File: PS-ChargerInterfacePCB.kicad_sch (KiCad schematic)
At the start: 32 parts, among them J2 LV_Elcon_Connector, J4 BPSConn, J5 Estop 2, J6 Estop 3, K2 Relay_SPST-NC

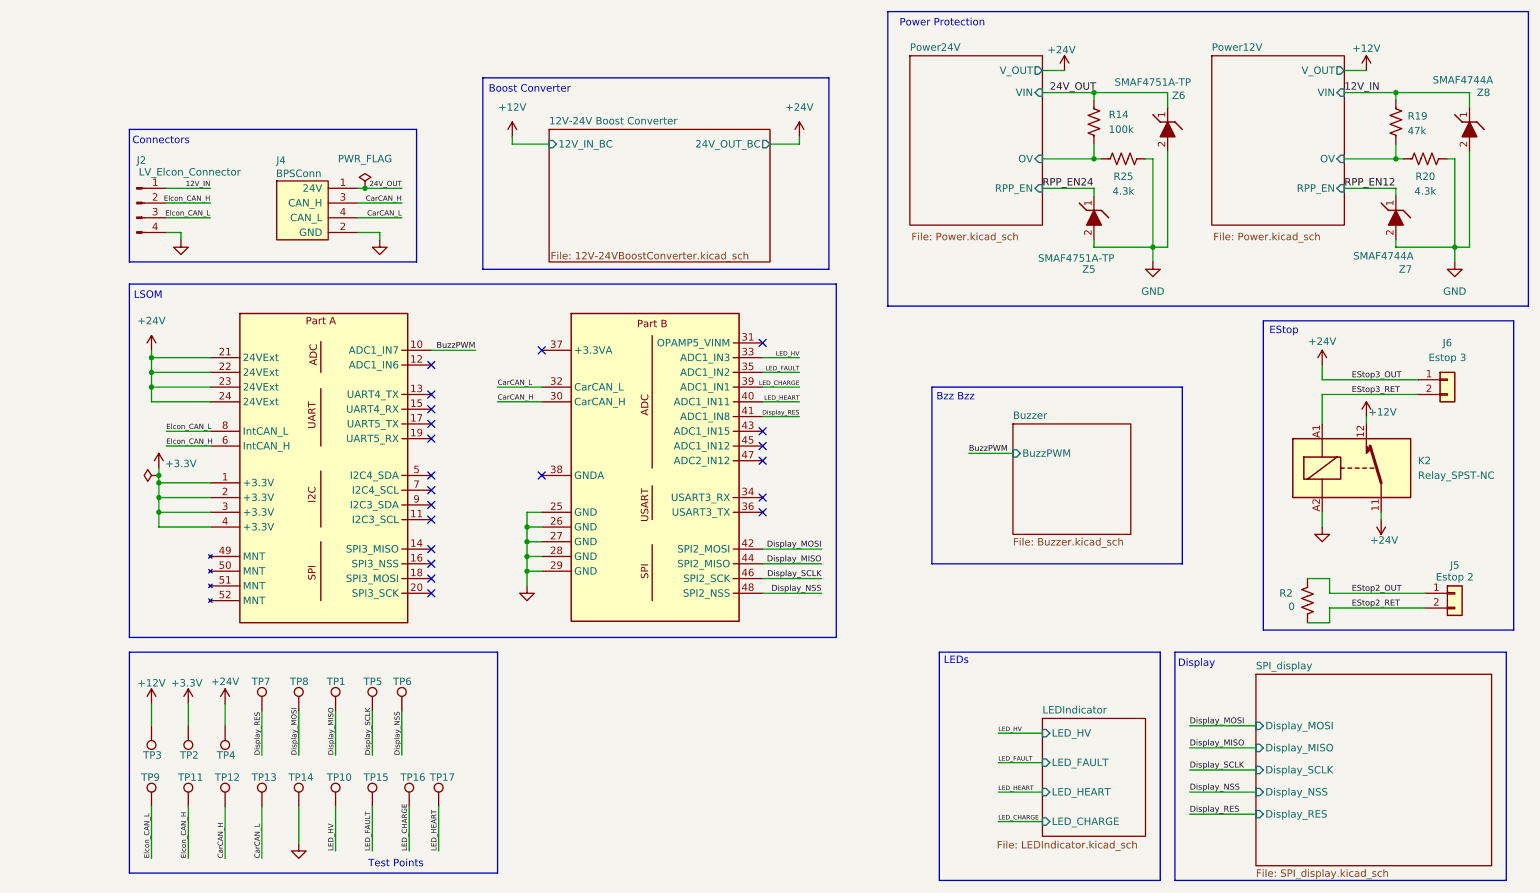
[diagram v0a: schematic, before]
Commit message: RevA5
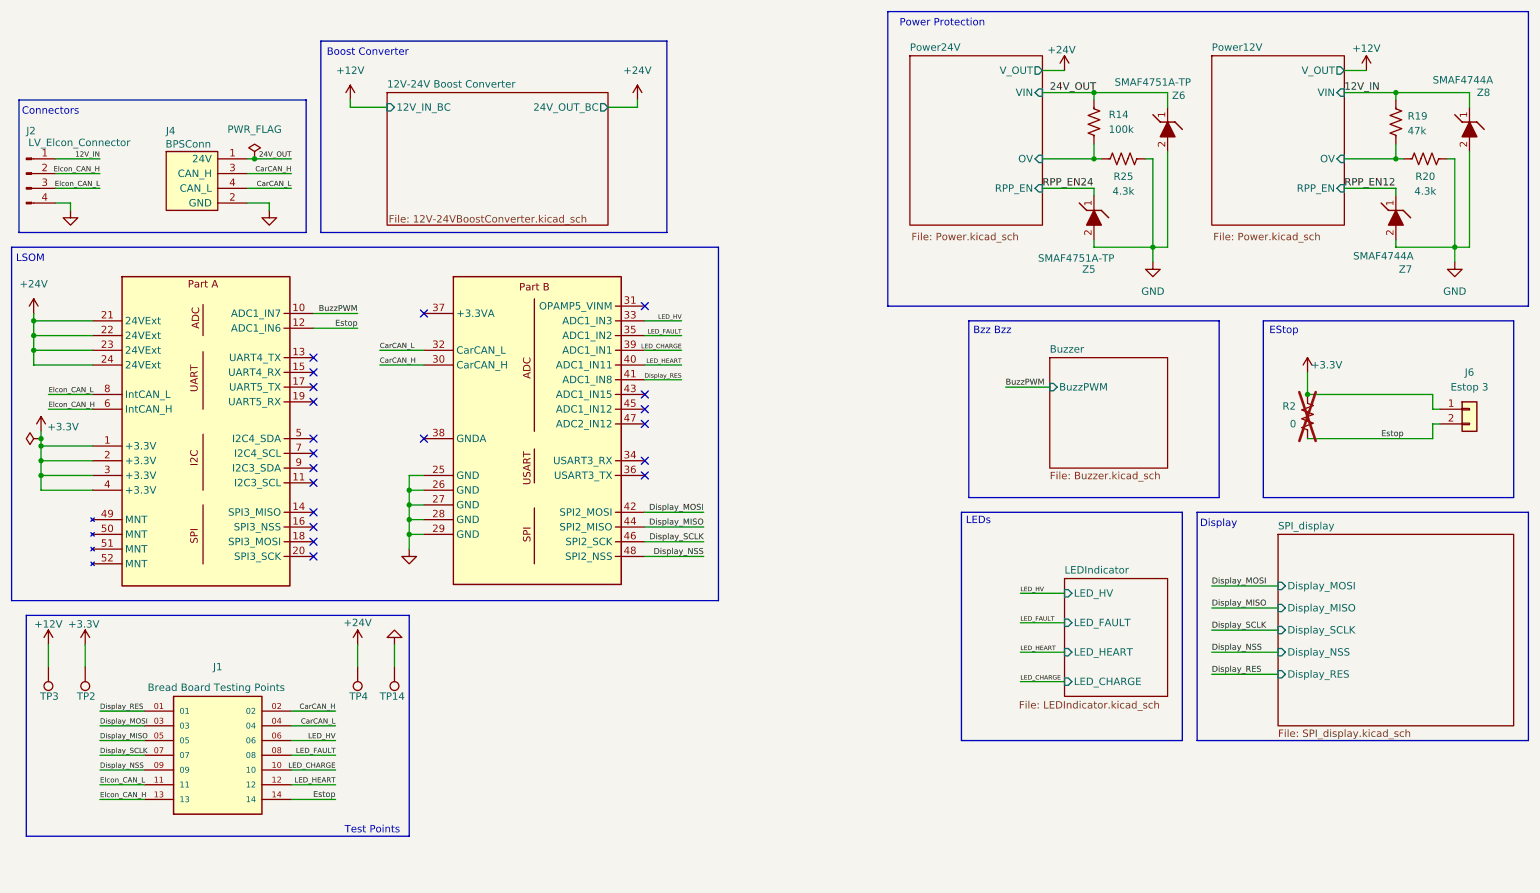
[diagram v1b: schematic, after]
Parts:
- removed J5: Estop 2, symbol Connector_Generic:Conn_01x02
- removed K2: Relay_SPST-NC, symbol Relay:Relay_SPST-NC
- removed TP1, TP10, TP11, TP12, TP13, TP15, TP16, TP17, TP5, TP6, TP7, TP8, TP9: TestPoint, symbol Connector:TestPoint
- added J1: Bread Board Testing Points, SSW-107-21-G-D:SAMTEC_SSW-107-21-G-D, symbol SSW-107-21-G-D:SSW-107-21-G-D
- R2: footprint (none) -> Resistor_SMD:R_0402_1005Metric; now not fitted
- TP14, TP2, TP3, TP4: footprint (none) -> UTSVT_Special:TestPoint_HEX_3mmID
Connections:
- net EStop2_OUT is gone; now on net +3.3V: R2.1
- net EStop2_RET is gone; now on net Estop: R2.2
- net EStop3_RET is gone; now on net Estop: J6.2 (Pin_2)
- net +24V: no longer J6.1 (Pin_1)
- net +3.3V: now also J6.1 (Pin_1)
- net CarCAN_H: now also J1.02
- net CarCAN_L: now also J1.04
- net Display_MISO: now also J1.05
- net Display_MOSI: now also J1.03
- net Display_NSS: now also J1.09
- net Display_RES: now also J1.01
- net Display_SCLK: now also J1.07
- net Elcon_CAN_H: now also J1.13
- net Elcon_CAN_L: now also J1.11
- net LED_CHARGE: now also J1.10
- net LED_FAULT: now also J1.08
- net LED_HEART: now also J1.12
- net LED_HV: now also J1.06
- net Estop: now reaches J3.12 (ADC1_IN6)
- net Estop: now also J1.14
- no-connect marks 21 -> 20
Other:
- moved on the sheet: J2, J4, J6, TP14, TP2, TP3, TP4
